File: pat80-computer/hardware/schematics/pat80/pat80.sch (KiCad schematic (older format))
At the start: 9 parts, among them SW1 SW_Push, U1 Z80CPU, U3 256k (32k x 8) EEPROM, U4 256k (32k x 8) SRAM

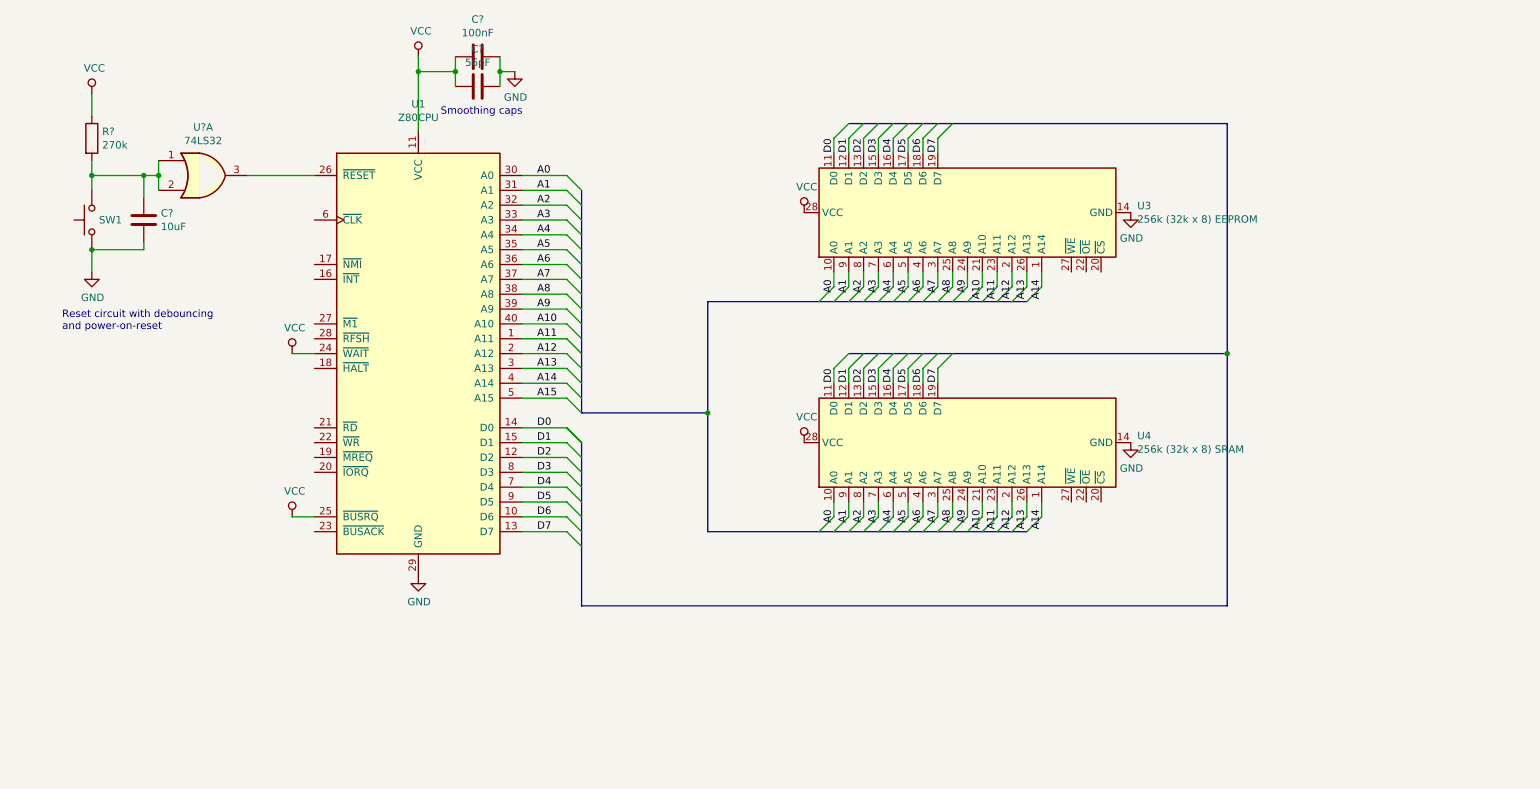
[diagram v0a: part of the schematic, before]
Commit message: WIP Schematics
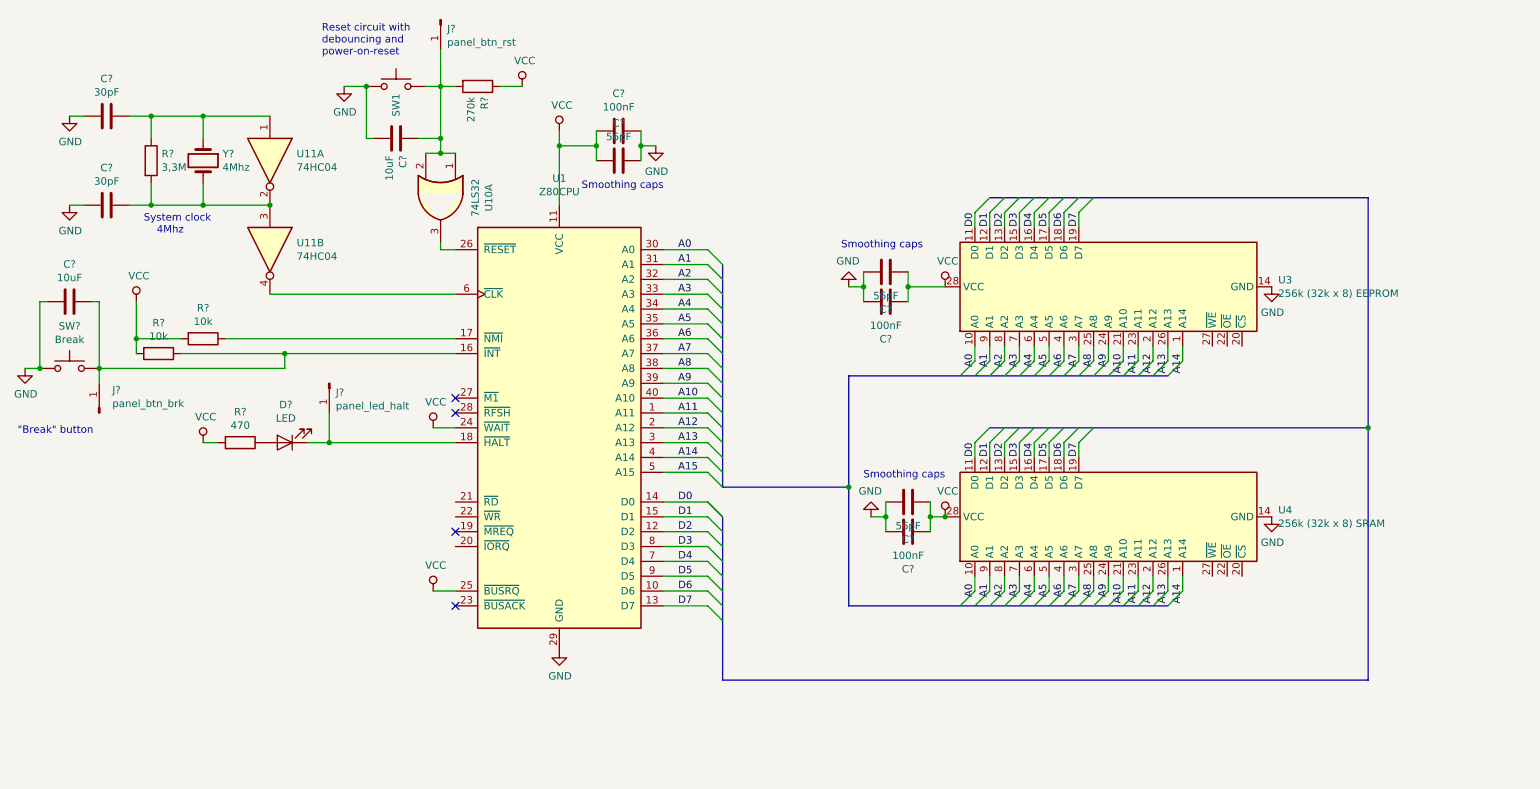
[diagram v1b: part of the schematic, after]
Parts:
- added C? (x2): 30pF, symbol Device:C
- added C? (x2): 100nF, symbol Device:C
- added C? (x2): 56pF, symbol Device:C
- added C?: 10uF, symbol Device:C
- added D?: LED, symbol Device:LED
- added J?: panel_btn_rst, symbol Connector:Conn_01x01_Male
- added J?: panel_btn_brk, symbol Connector:Conn_01x01_Male
- added J?: panel_led_halt, symbol Connector:Conn_01x01_Male
- added R?: 3,3M, symbol Device:R
- added R? (x2): 10k, symbol Device:R
- added R?: 470, symbol Device:R
- added SW?: Break, symbol Switch:SW_Push
- added U11: 74HC04, symbol 74xx:74HC04
- added Y?: 4Mhz, symbol Device:Crystal
- gave numbers to parts that had none: 1
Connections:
- net GND: now also C?.1, C?.1, C?.1, C?.1, C?.2, C?.2, C?.2, SW?.1
- net VCC: now also C?.2, C?.2, C?.2, C?.2, R?.2, R?.2, R?.2
- net at U1.16 (~INT~): now also C?.1, J?.1 (Pin_1), R?.1, SW?.2
- net at U1.17 (~NMI~): now also R?.1
- net at U1.18 (~HALT~): now also D?.1 (K), J?.1 (Pin_1)
- net at U1.6 (~CLK~): now also U11.4
- net at C?.1, R?.2, SW1.2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: now also J?.1 (Pin_1)
- new net: C?.1, R?.1, U11.1, Y?.1
- new net: C?.1, R?.2, U11.2, U11.3, Y?.2
- new net: D?.2 (A), R?.1
- no-connect marks 0 -> 4
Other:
- note added: ""Break" button"
- note added: "Reset circuit with\ndebouncing and\npower-on-reset"
- note added: "System clock\n 4Mhz"
- note removed: "Reset circuit with debouncing\nand power-on-reset"
- moved on the sheet: C?, R?, SW1, U1, U10A, U3, U4
